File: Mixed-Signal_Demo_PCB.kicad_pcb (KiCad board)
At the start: 4 copper layers, 60 x 75 mm, 114 parts, among them J301 USB_C_Receptacle_USB2.0_16P, J302 2x5x1.27mm, J401 DOSIN-801-0031, J501 DOSIN-801-0031, U201 HT7533-1, U202 MCP6001T-E/OT, U203 TLV62569DBV, U301 STM32F103CBTx, U302 USBLC6-2SC6, U401 MCP6001T-E/OT, U402 MCP6001T-E/OT, U403 ADC141S626CIMM_NOPB, U404 REF3033A/DBZT, U501 MCP6001T-E/OT, U502 DAC7563TDGSR, Y301 16MHz

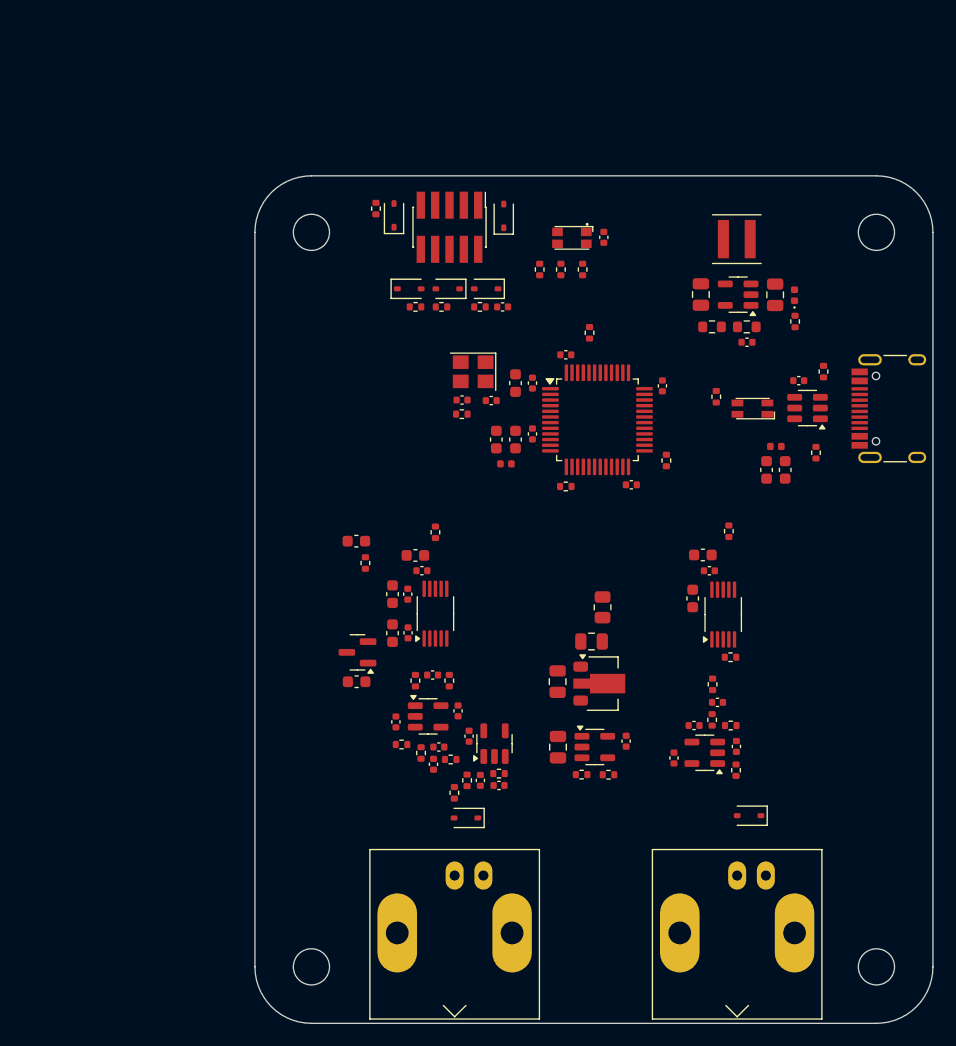
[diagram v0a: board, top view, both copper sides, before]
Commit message: Lesson 13: Routing
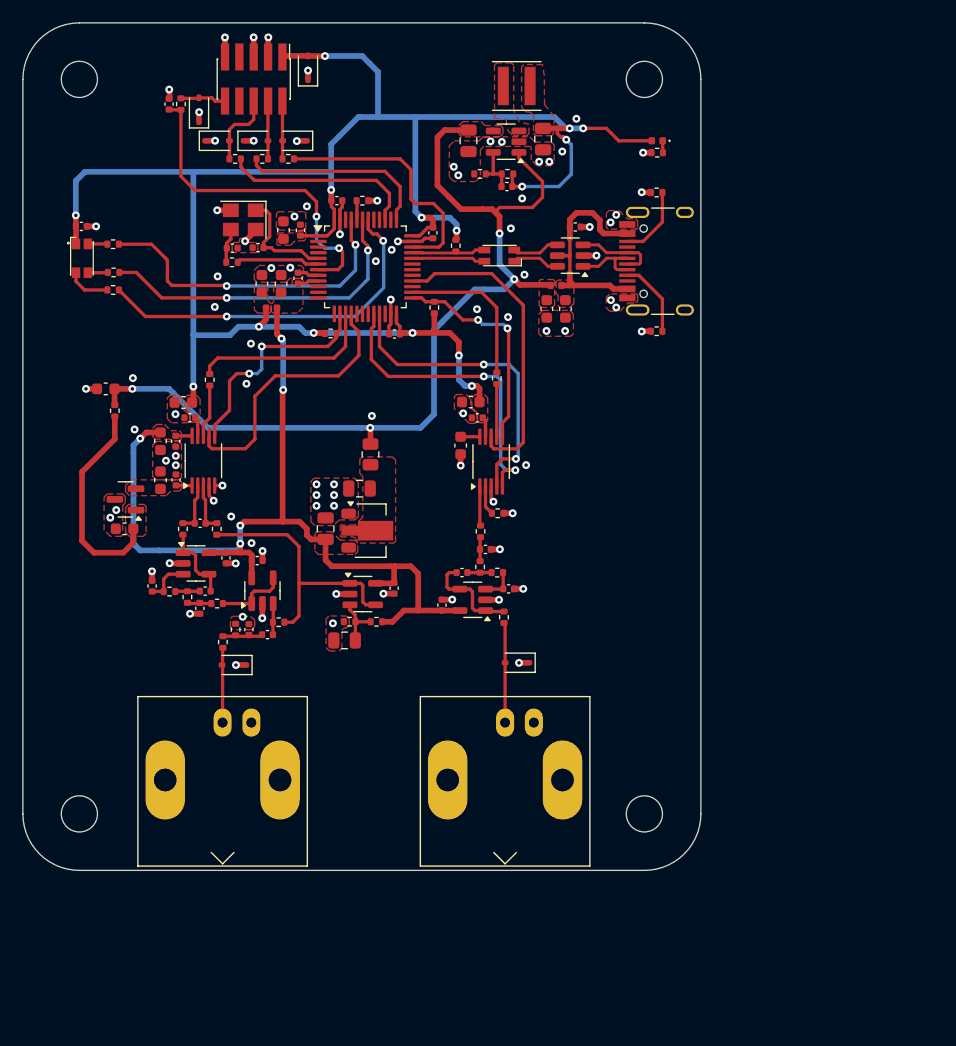
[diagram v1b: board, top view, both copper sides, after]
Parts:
- R204, R206: footprint Resistor_SMD:R_0603_1608Metric -> Resistor_SMD:R_0402_1005Metric
- moved C312 46.2 mm to (91.1, 77.5), turned to 0 degrees
- moved D301 43.4 mm to (91.2, 80.3), turned to 90 degrees
- moved R308 41.6 mm to (94.0, 79.0), turned to 180 degrees
- moved R313 39.6 mm to (94.0, 81.5), turned to 180 degrees
- moved R310 37.8 mm to (94.0, 83.1), turned to 180 degrees
- moved C313 34.5 mm to (98.9, 66.7), turned to 90 degrees
- moved R314 32.0 mm to (100.0, 66.7), turned to -90 degrees
- moved D306 29.9 mm to (101.5, 67.2), turned to 90 degrees
- moved R306 26.6 mm to (124.3, 79.2)
- moved FL301 26.2 mm to (128.1, 80.1)
- moved R409 25.9 mm to (94.1, 93.8)
- moved C413 25.9 mm to (93.3, 91.9)
- moved C209 25.3 mm to (128.8, 74.0)
- moved R204 25.1 mm to (128.8, 72.8)
- moved U302 25.0 mm to (134.4, 80.1)
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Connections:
- net /Power/BUCK_5W renamed /Power/BUCK_SW
- J302 pad 10: /MCU/SWDIO_CONN -> /MCU/NRST_CONN
- J302 pad 2: GND -> /MCU/SWDIO_CONN
- J302 pad 4: unconnected-(J302-Pin_4-Pad4) -> /MCU/SWCLK_CONN
- J302 pad 6: /MCU/NRST_CONN -> /MCU/SWO_CONN
- J302 pad 8: /MCU/SWO_CONN -> unconnected-(J302-Pin_8-Pad8)
- J302 pad 9: /MCU/SWCLK_CONN -> GND
- R308 pad 1: /MCU/TIM4_CH1 -> /MCU/TIM4_CH3
- R310 pad 1: /MCU/TIM4_CH2 -> /MCU/TIM4_CH1
- R313 pad 1: /MCU/TIM4_CH3 -> /MCU/TIM4_CH2
- U301 pad 20: unconnected-(U301-PB2-Pad20) -> DAC_NCLR
- U301 pad 21: DAC_NCLR -> DAC_NLDAC
- U301 pad 22: DAC_NLDAC -> unconnected-(U301-PB11-Pad22)
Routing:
- net +3.3V: track 0.00 -> 177.4 mm, vias 0 -> 15
- net +3.3VA: track 0.00 -> 85.3 mm, vias 0 -> 5
- net +5V: track 0.00 -> 82.5 mm, vias 0 -> 4
- net GND: track 0.00 -> 50.2 mm, vias 0 -> 91
- net /MCU/TIM4_CH1: track 0.00 -> 32.3 mm, vias 0 -> 2
- net /MCU/NRST: track 0.00 -> 29.4 mm, vias 0 -> 2
- net /MCU/TIM4_CH2: track 0.00 -> 29.1 mm, vias 0 -> 2
- net /MCU/TIM4_CH3: track 0.00 -> 28.7 mm, vias 0 -> 2
- net DAC_NCLR: track 0.00 -> 27.8 mm, vias 0 -> 2
- net DAC_NLDAC: track 0.00 -> 27.6 mm, vias 0 -> 2
- net SPI2_MOSI: track 0.00 -> 27.4 mm
- net SPI1_MISO: track 0.00 -> 23.9 mm
- net VCOM: track 0.00 -> 23.8 mm
- net /MCU/SWDIO: track 0.00 -> 22.2 mm
- net SPI1_NSS: track 0.00 -> 19.9 mm, vias 0 -> 2
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- added copper zone on F.Cu, net +3.3V
- added copper zone on F.Cu, net +3.3VA
- added copper zone on F.Cu, net +5V
- added copper zone on F.Cu, net /ADC/ADC_REF_IN
- added copper zone on F.Cu, net /ADC/ADC_VREF
- added copper zone on F.Cu, net /Power/+5V_FILT
- added copper zone on F.Cu, net /Power/BUCK_SW
- added copper zone on F.Cu, net GND
- added copper zone on In1.Cu, net GND
- added copper zone on In2.Cu, net GND
- added copper zone on F.Cu, net VBUS
